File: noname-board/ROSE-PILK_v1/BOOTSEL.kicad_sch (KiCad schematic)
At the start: 3 parts

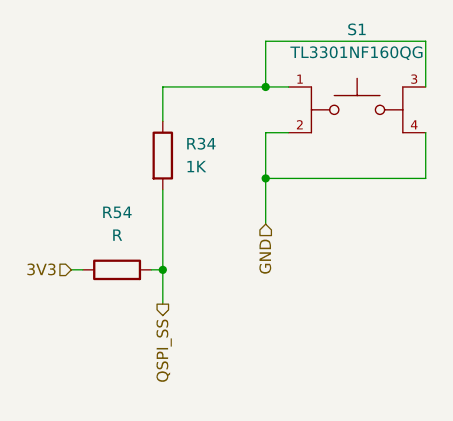
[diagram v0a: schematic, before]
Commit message: Ben
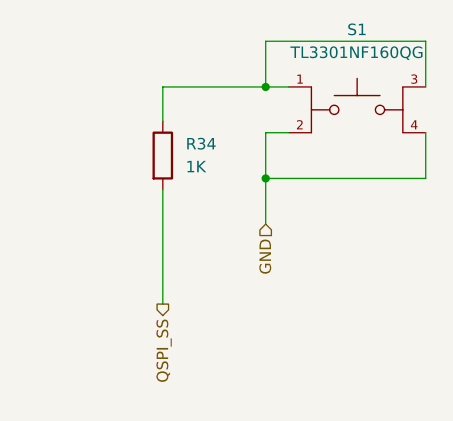
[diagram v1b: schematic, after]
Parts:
- removed R54: R, Resistor_THT:R_Axial_DIN0207_L6.3mm_D2.5mm_P10.16mm_Horizontal, symbol Device:R
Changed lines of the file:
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@@
   (junction (at 134.62 60.96) (diameter 0) (color 0 0 0 0)
   )
-  (junction (at 123.19 71.12) (diameter 0) (color 0 0 0 0)
-  )
   (wire (pts (xy 123.19 54.61) (xy 123.19 50.8))
-    (stroke (width 0) (type default))
-  )
-  (wire (pts (xy 121.92 71.12) (xy 123.19 71.12))
     (stroke (width 0) (type default))
   )
@@
     (stroke (width 0) (type default))
   )
-  (wire (pts (xy 123.19 62.23) (xy 123.19 71.12))
-    (stroke (width 0) (type default))
-  )
-  (wire (pts (xy 123.19 71.12) (xy 123.19 74.93))
+  (wire (pts (xy 123.19 62.23) (xy 123.19 74.93))
     (stroke (width 0) (type default))
   )
@@
     (stroke (width 0) (type default))
   )
-  (wire (pts (xy 113.03 71.12) (xy 114.3 71.12))
-    (stroke (width 0) (type default))
-  )
   (wire (pts (xy 134.62 45.72) (xy 134.62 50.8))
     (stroke (width 0) (type default))
@@
   )
   (hierarchical_label "GND" (shape input) (at 134.62 66.04 270) (fields_autoplaced)
-    (effects (font (size 1.27 1.27)) (justify right))
-  )
-  (hierarchical_label "3V3" (shape input) (at 113.03 71.12 180) (fields_autoplaced)
     (effects (font (size 1.27 1.27)) (justify right))
   )
@@
         )
       )
-    )
-  )
-  (symbol (lib_id "Device:R") (at 118.11 71.12 90) (unit 1)
-    (in_bom yes) (on_board yes) (dnp no) (fields_autoplaced)
-    (property "Reference" "R54" (at 118.11 64.77 90)
-      (effects (font (size 1.27 1.27)))
-    )
-    (property "Value" "R" (at 118.11 67.31 90)
-      (effects (font (size 1.27 1.27)))
-    )
-    (property "Footprint" "Resistor_THT:R_Axial_DIN0207_L6.3mm_D2.5mm_P10.16mm_Horizontal" (at 118.11 72.898 90)
-      (effects (font (size 1.27 1.27)) hide)
-    )
-    (property "Datasheet" "~" (at 118.11 71.12 0)
-      (effects (font (size 1.27 1.27)) hide)
-    )
-    (pin "1")
-    (pin "2")
-    (instances
-      (project "ROSE-PILK_v1"
-        (path "/3dfb9737-68ba-4ca9-8085-72e4f57f9e50/ee4b99aa-294b-4c3b-9b79-fbaf11f9a74b"
-          (reference "R54") (unit 1)
-        )
-        (path "/3dfb9737-68ba-4ca9-8085-72e4f57f9e50/853a186f-a31e-46ca-9745-e888a8f62939"
-          (reference "R55") (unit 1)
-        )
-      )
